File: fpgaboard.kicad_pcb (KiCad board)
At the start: 2 copper layers, 110.6 x 80.3 mm, 45 parts, among them J1 Conn_02x06_Odd_Even, J2 Conn_02x06_Odd_Even, J3 Conn_02x06_Odd_Even, J4 Conn_02x06_Odd_Even, J5 Conn_02x06_Odd_Even, J6 Conn_02x06_Odd_Even, J7 Conn_02x20_Odd_Even, U1 ICE40HX4K-TQ144, U2 TLV73312PDBV, U3 TLV73333PDBV

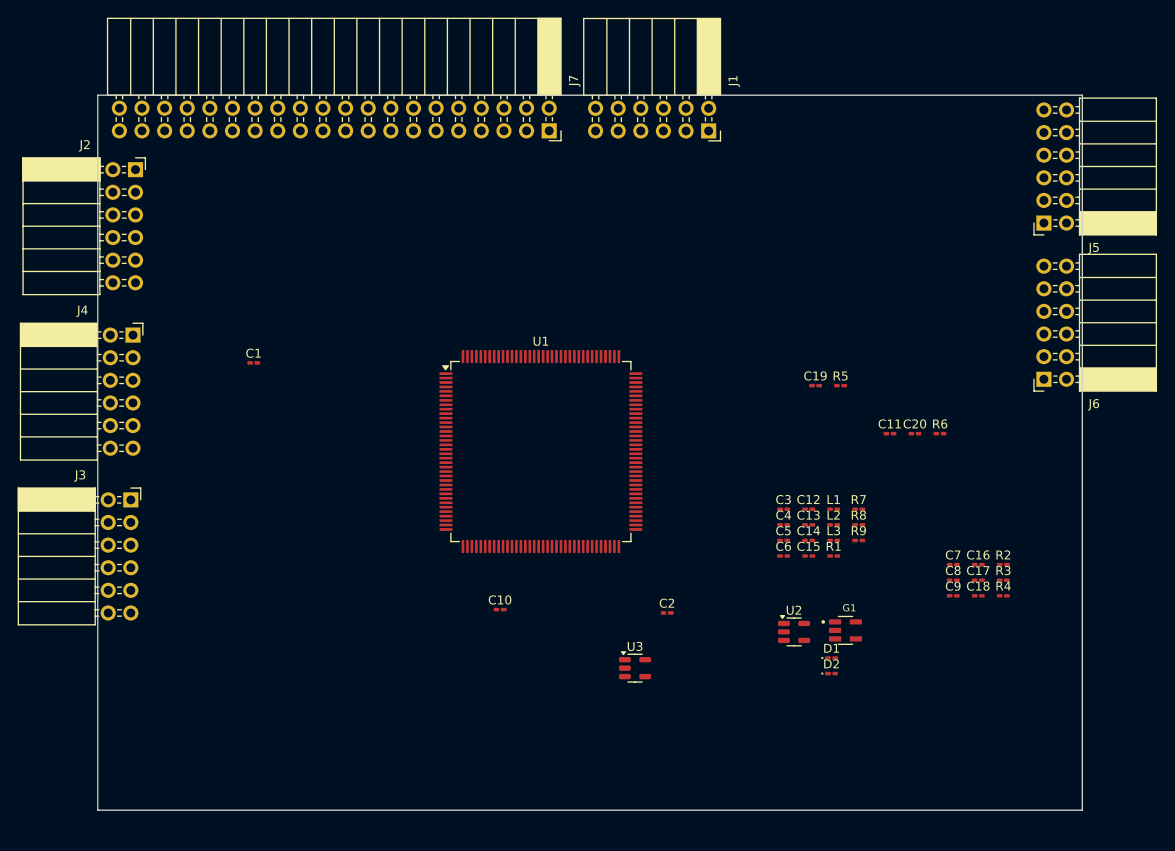
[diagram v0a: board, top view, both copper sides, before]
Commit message: fpgaboard
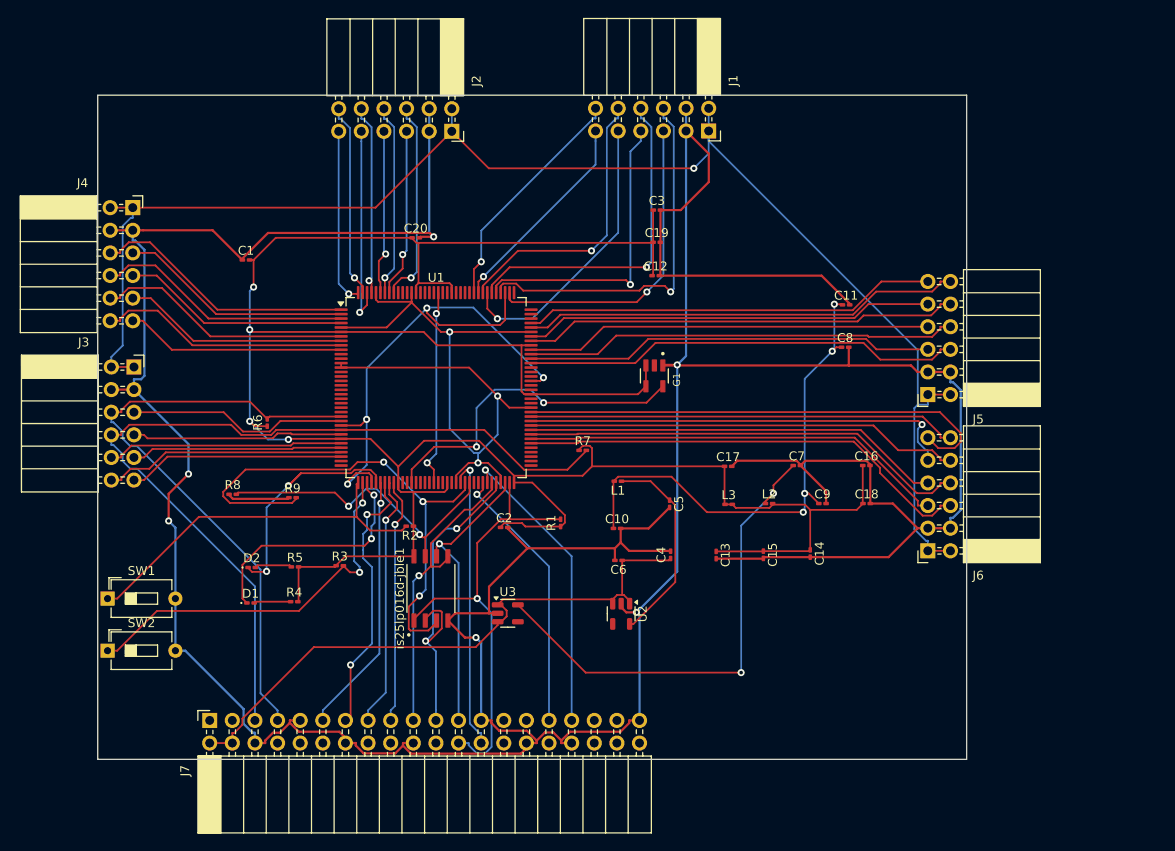
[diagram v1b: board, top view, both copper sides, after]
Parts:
- added SW1: SW_Push, Button_Switch_THT:SW_DIP_SPSTx01_Slide_6.7x4.1mm_W7.62mm_P2.54mm_LowProfile, F.Cu at (93.4, 120.2)
- added SW2: SW_Push, Button_Switch_THT:SW_DIP_SPSTx01_Slide_6.7x4.1mm_W7.62mm_P2.54mm_LowProfile, F.Cu at (93.4, 126.0)
- added is25lp016d-jble1: ~, flash:SOIC127P790X216-8N, F.Cu at (129.7, 119.0)
- moved R4 79.6 mm to (114.3, 120.5)
- moved J7 76.4 mm to (104.8, 133.8), turned to 90 degrees
- moved R6 75.5 mm to (111.3, 100.4), turned to 90 degrees
- moved R3 74.5 mm to (119.5, 116.5)
- moved R8 70.4 mm to (107.4, 108.5)
- moved R2 66.8 mm to (127.3, 112.0), turned to 180 degrees
- moved D2 66.2 mm to (109.6, 116.7)
- moved D1 65.5 mm to (109.4, 120.7)
- moved R5 64.6 mm to (114.4, 116.6)
- moved R9 63.8 mm to (114.2, 108.8)
- moved C20 60.2 mm to (128.0, 79.7)
- moved C3 36.5 mm to (155.1, 76.5)
- moved J2 35.8 mm to (132.0, 67.7), turned to -90 degrees
- moved G1 35.7 mm to (154.8, 95.2), turned to -90 degrees
- moved R7 31.7 mm to (146.7, 103.5)
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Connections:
- J1 pad 10: /p1_8 -> /p1_2
- J1 pad 11: /p1_1 -> /p1_7
- J1 pad 12: /p1_7 -> /p1_1
- J1 pad 5: /p1_4 -> /p1_10
- J1 pad 6: /p1_10 -> /p1_4
- J1 pad 7: /p1_3 -> /p1_9
- J1 pad 8: /p1_9 -> /p1_3
- J1 pad 9: /p1_2 -> /p1_8
- J7 pad 11: /cdone -> /gp16
- J7 pad 13: /creset -> /gp13
- J7 pad 15: /gp22 -> /gp12
- J7 pad 17: /pi_3v3_2 -> /gp6
- J7 pad 27: /gp0 -> /gp3
- J7 pad 29: /gp5 -> /gp4
- J7 pad 31: /gp6 -> /cdone
- J7 pad 32: /gp12 -> /gp22
- J7 pad 33: /gp13 -> /creset
- J7 pad 36: /gp16 -> /pi_3v3_2
- J7 pad 38: /gp20 -> /gp0
- J7 pad 40: /gp21 -> /gp5
- J7 pad 5: /gp3 -> /gp20
- J7 pad 7: /gp4 -> /gp21
- R8 pad 2: /sd1o3 -> /sd_io3
- R9 pad 2: /sd1o2 -> /sd_io2
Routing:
- net GND: track 0.00 -> 478.3 mm, vias 0 -> 6
- net +3.3V: track 0.00 -> 292.3 mm, vias 0 -> 4
- net +3.3VP: track 0.00 -> 167.4 mm, vias 0 -> 1
- net /gp20: track 0.00 -> 96.8 mm
- net Net-(U1E-GND-Pad103): track 0.00 -> 85.0 mm, vias 0 -> 3
- net /gp21: track 0.00 -> 70.3 mm
- net +5V: track 0.00 -> 68.2 mm
- net Net-(U1E-VCC-Pad111): track 0.00 -> 61.9 mm, vias 0 -> 4
- net /sd_io2: track 0.00 -> 60.0 mm, vias 0 -> 3
- net +1V2: track 0.00 -> 57.5 mm, vias 0 -> 4
- net Net-(U3-OUT): track 0.00 -> 55.4 mm, vias 0 -> 2
- net /p6_1: track 0.00 -> 54.7 mm
- net /p6_10: track 0.00 -> 51.6 mm
- net /gp8: track 0.00 -> 51.0 mm, vias 0 -> 1
- net /p6_9: track 0.00 -> 50.5 mm
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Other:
- board size 110.6 x 80.3 mm -> 97.6 x 74.6 mm
